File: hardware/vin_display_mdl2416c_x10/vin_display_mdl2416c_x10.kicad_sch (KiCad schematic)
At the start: 52 parts, among them J1 DEBUG, J2 USB_B_Micro, J3 DEBUG_UART, J4 IF_UART, J5 AUX_CONNECTOR, Q1 BSS138, SW1 SW_RESET, SW2 BOOTSEL, SW3 KNOB, U1 W25Q16JVSNIQ, U2 MIC23050-SYML, U3 RP2040, U4 HEF4028BT, X1 12MHz

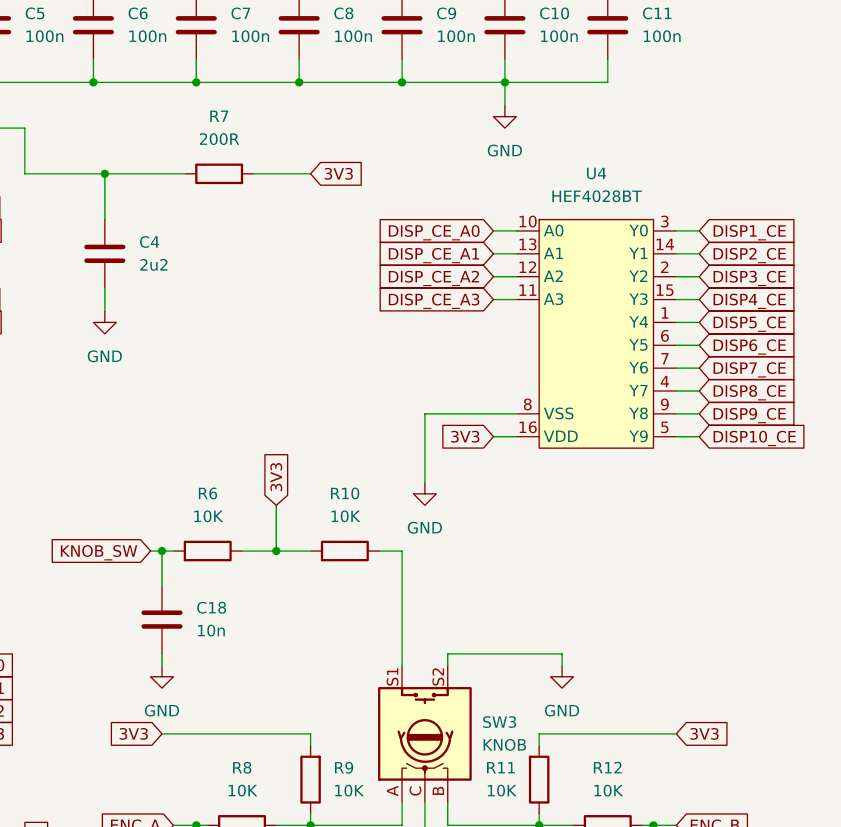
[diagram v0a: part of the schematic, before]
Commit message: update schematic; add pdf
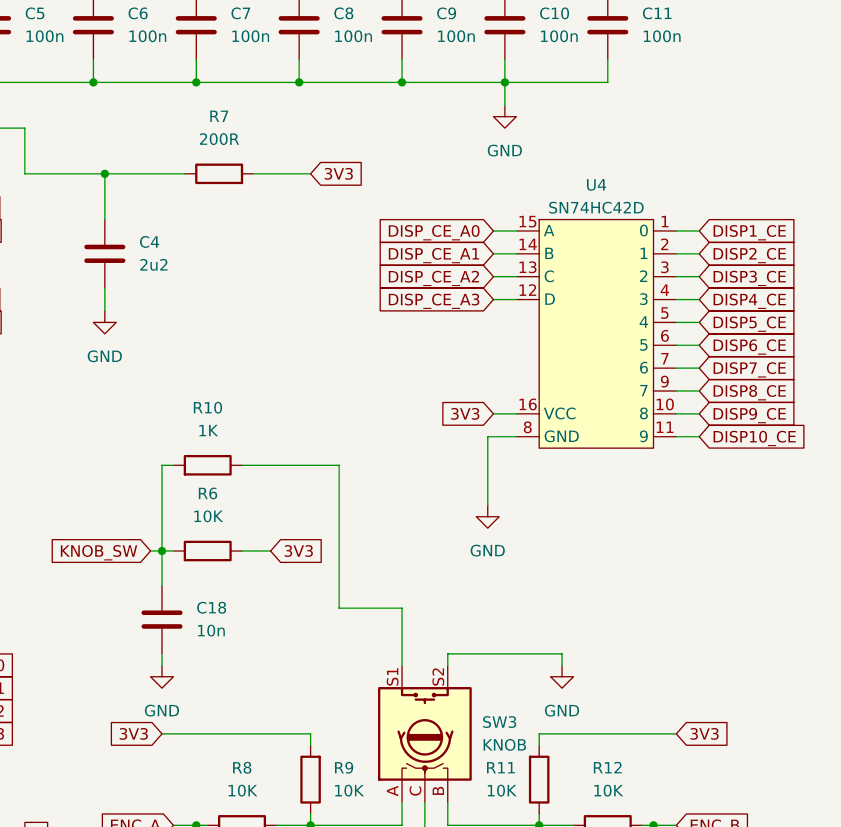
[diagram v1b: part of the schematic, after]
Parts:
- removed U4: HEF4028BT, components:SO16, symbol components:HEF4028BT
- added U4: SN74HC42D, components:SO16, symbol components:SN74HC42D
- R10: value 10K -> 1K
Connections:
- net 3V3: now also U4.16 (VCC); no longer R10.2
- net DISP10_CE: now also U4.11 (9)
- net DISP1_CE: now also U4.1 (0)
- net DISP2_CE: now also U4.2 (1)
- net DISP3_CE: now also U4.3 (2)
- net DISP4_CE: now also U4.4 (3)
- net DISP5_CE: now also U4.5 (4)
- net DISP6_CE: now also U4.6 (5)
- net DISP7_CE: now also U4.7 (6)
- net DISP8_CE: now also U4.9 (7)
- net DISP9_CE: now also U4.10 (8)
- net DISP_CE_A0: now also U4.15 (A)
- net DISP_CE_A1: now also U4.14 (B)
- net DISP_CE_A2: now also U4.13 (C)
- net DISP_CE_A3: now also U4.12 (D)
- net GND: now also U4.8 (GND)
- net KNOB_SW: now also R10.2
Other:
- moved on the sheet: R10
